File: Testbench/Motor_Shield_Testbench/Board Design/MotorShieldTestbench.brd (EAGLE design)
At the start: 63.5 x 87.6 mm, 49 parts, among them IC2 74LS04D, IC3 74AC74D, IC4 74AC74D, U1 ATMEGA2560AU, U10 +12v, U2 FT232RL, U3 ATTINY85-20SU, U4 ATTINY85-20SU, U6 SN74LVC2G157DCTR, U7 SN74LVC2G157DCTR, U8 SN74LVC2G157DCTR, U9 SN74LVC2G157DCTR, X4 2510-, X5 2510-, X6 MINI-USB_4P-32005-101

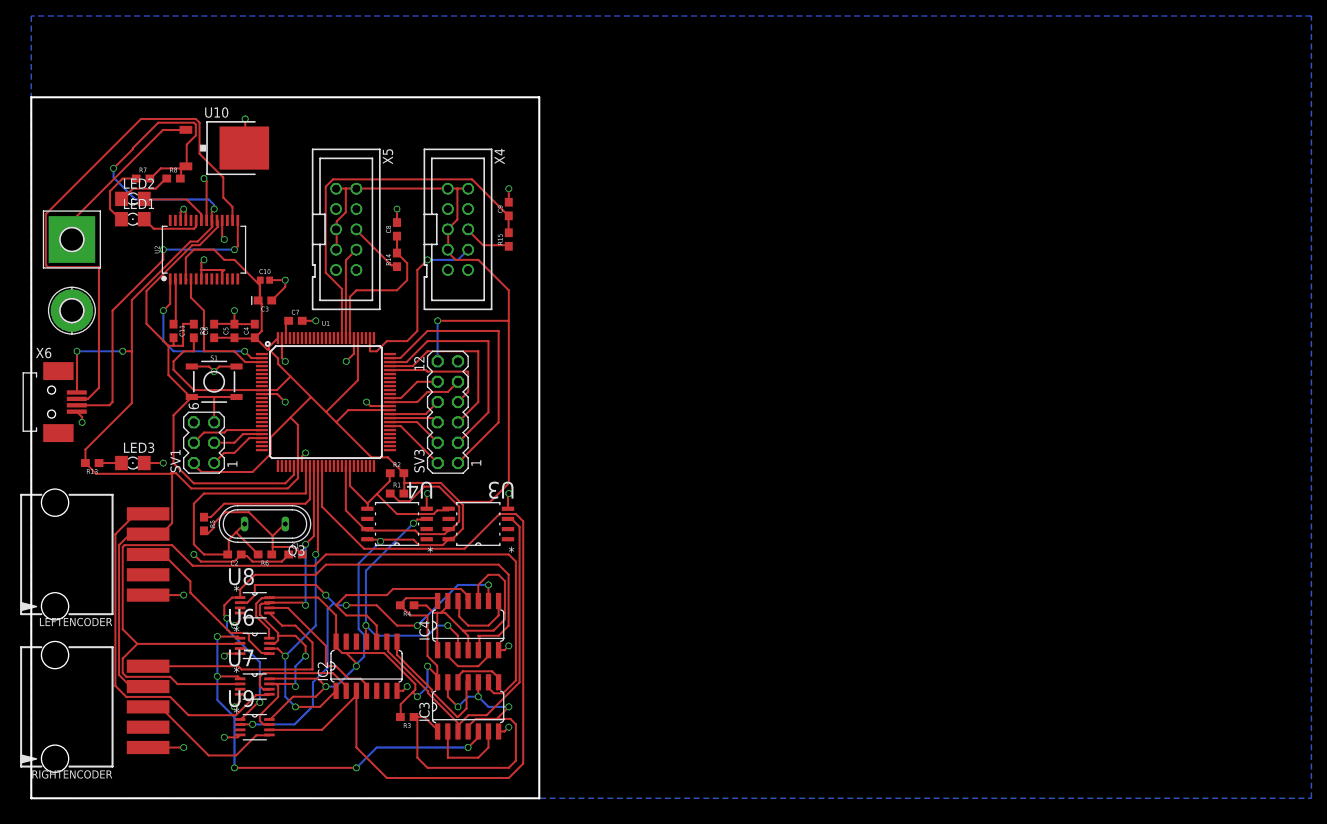
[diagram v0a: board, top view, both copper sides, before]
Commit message: minor improvements
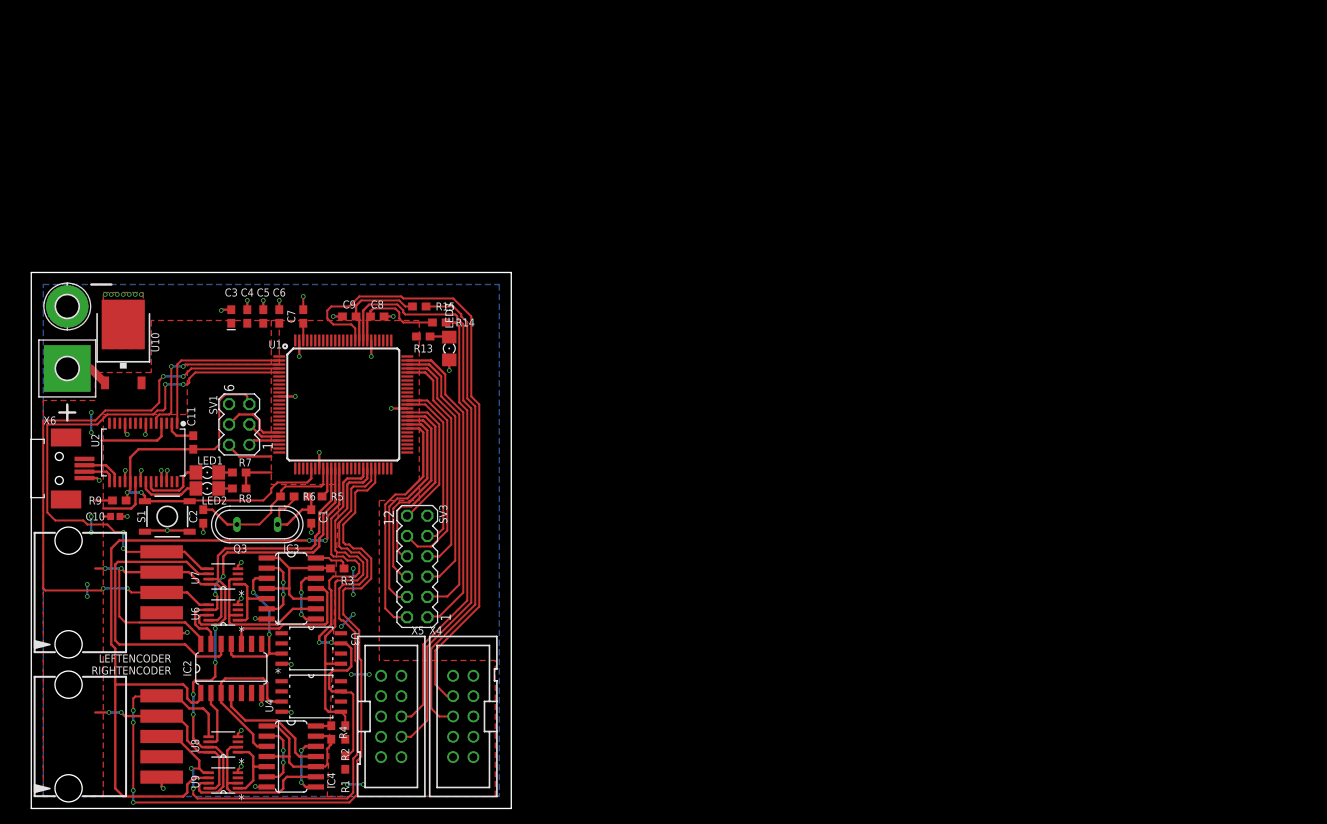
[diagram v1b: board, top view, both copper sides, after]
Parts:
- moved X5 61.1 mm to (45.0, 11.5)
- moved X4 60.9 mm to (54.0, 11.5), turned to 90 degrees
- moved R13 44.3 mm to (49.0, 59.0)
- moved LED3 42.1 mm to (52.2, 57.5), turned to 270 degrees
- moved R8 39.6 mm to (26.0, 40.0)
- moved R7 38.7 mm to (26.0, 42.0)
- moved LED2 37.4 mm to (22.0, 40.0), turned to 180 degrees
- moved C10 35.0 mm to (10.5, 36.5)
- moved R1 34.2 mm to (39.2, 5.75), turned to 270 degrees
- moved R2 33.0 mm to (39.2, 9.50), turned to 270 degrees
- moved LED1 33.0 mm to (22.0, 42.0), turned to 180 degrees
- moved U10 27.6 mm to (11.5, 58.0), turned to 0 degrees
- moved IC4 27.5 mm to (32.5, 6.50), turned to 270 degrees
- moved IC3 26.6 mm to (32.5, 27.5), turned to 270 degrees
- moved U2 26.5 mm to (14.0, 44.5), turned to 180 degrees
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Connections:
- net LE1: now also U1.4
- net LE2: now also U1.5
- net LSELECT: now also IC2.13; no longer IC2.1
- net LWAVE: now also IC2.11; no longer IC2.9
- net N$14: now also IC2.4; no longer IC2.10
- net N$27: now also IC2.10; no longer IC2.8
- net N$3: now also IC2.2; no longer IC2.4
- net N$8: now also IC2.12; no longer IC2.2
- net RDIR: now also U1.85; no longer U1.77
- net RE1: now also U1.45
- net RE2: now also U1.46
- net RSELECT: now also IC2.1; no longer IC2.3
- net RWAVE: now also IC2.3; no longer IC2.11
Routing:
- net +5V: track 500.6 -> 134.5 mm, vias 10 -> 18
- net LWAVE2: track 116.6 -> 19.2 mm
- net RE2: track 31.3 -> 106.8 mm, vias 0 -> 4
- net D-: track 69.8 -> 5.20 mm
- net RE1: track 18.8 -> 82.7 mm, vias 0 -> 2
- net LDIR: track 11.7 -> 74.2 mm
- net RWAVE1: track 68.7 -> 9.14 mm, vias 2 -> 0
- net LE1: track 21.6 -> 76.5 mm, vias 0 -> 4
- net RDIR: track 23.7 -> 77.8 mm, vias 1 -> 0
- net RSPEEDH: track 6.08 -> 60.2 mm
- net LSPEEDH: track 7.15 -> 55.2 mm
- net GND: track 102.6 -> 55.0 mm, vias 30 -> 42
- net LWAVE1: track 56.2 -> 8.98 mm, vias 5 -> 0
- net RWAVE2: track 63.5 -> 20.3 mm, vias 5 -> 0
- net RSPEED: track 47.0 -> 12.1 mm
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- added copper zone on layer 1, net +5V
- added copper zone on layer 1, net GND
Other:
- board size 63.5 x 87.6 mm -> 60 x 67 mm
- board text added: "MotorShieldTestbench Example Routing"
